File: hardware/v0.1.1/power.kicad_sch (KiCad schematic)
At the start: 5 parts

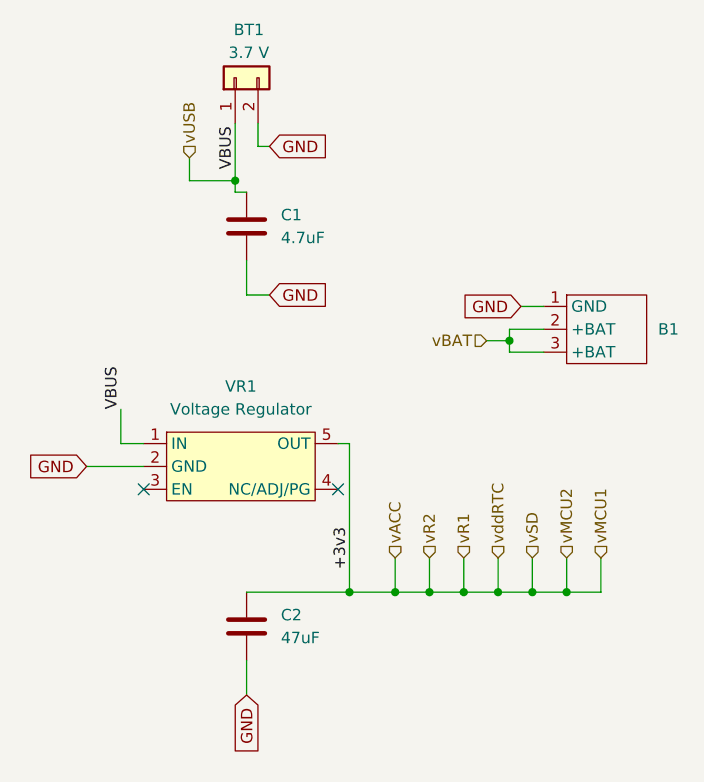
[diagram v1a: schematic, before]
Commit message: Pin updates and power fixes
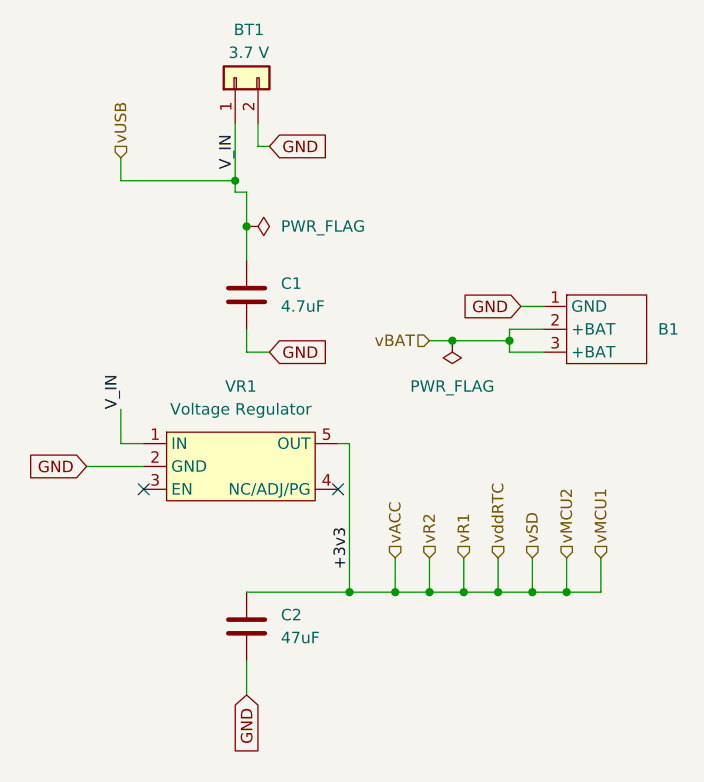
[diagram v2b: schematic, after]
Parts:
- VR1: symbol Device:Variable_Resistor -> PATCH_sym_2:Variable_Resistor
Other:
- moved on the sheet: C1
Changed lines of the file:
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@@
+	)
+	(junction
+		(at 165.1 93.98)
+		(diameter 0)
+		(color 0 0 0 0)
 	)
 	(junction
@@
 	)
 	(junction
+		(at 142.24 81.28)
+		(diameter 0)
+		(color 0 0 0 0)
+	)
+	(junction
 		(at 171.45 93.98)
 		(diameter 0)
@@
 	(wire
 		(pts
-			(xy 168.91 93.98) (xy 171.45 93.98)
-		)
-		(stroke
-			(width 0)
-			(type default)
-		)
-	)
-	(wire
-		(pts
-			(xy 142.24 88.9) (xy 144.78 88.9)
+			(xy 165.1 93.98) (xy 171.45 93.98)
 		)
 		(stroke
@@
 	(wire
 		(pts
+			(xy 142.24 81.28) (xy 142.24 85.09)
+		)
+		(stroke
+			(width 0)
+			(type default)
+		)
+	)
+	(wire
+		(pts
 			(xy 171.45 92.71) (xy 175.26 92.71)
 		)
@@
 	(wire
 		(pts
-			(xy 135.89 76.2) (xy 140.97 76.2)
-		)
-		(stroke
-			(width 0)
-			(type default)
-		)
-	)
-	(wire
-		(pts
 			(xy 170.18 118.11) (xy 170.18 121.92)
 		)
@@
 	(wire
 		(pts
+			(xy 142.24 95.25) (xy 144.78 95.25)
+		)
+		(stroke
+			(width 0)
+			(type default)
+		)
+	)
+	(wire
+		(pts
 			(xy 128.27 101.6) (xy 128.27 105.41)
 		)
@@
 	(wire
 		(pts
+			(xy 142.24 77.47) (xy 142.24 81.28)
+		)
+		(stroke
+			(width 0)
+			(type default)
+		)
+	)
+	(wire
+		(pts
 			(xy 177.8 121.92) (xy 181.61 121.92)
 		)
@@
 	(wire
 		(pts
+			(xy 128.27 76.2) (xy 140.97 76.2)
+		)
+		(stroke
+			(width 0)
+			(type default)
+		)
+	)
+	(wire
+		(pts
 			(xy 171.45 95.25) (xy 171.45 93.98)
 		)
@@
 	(wire
 		(pts
-			(xy 135.89 73.66) (xy 135.89 76.2)
-		)
-		(stroke
-			(width 0)
-			(type default)
-		)
-	)
-	(wire
-		(pts
 			(xy 171.45 93.98) (xy 171.45 92.71)
 		)
@@
 	(wire
 		(pts
-			(xy 142.24 85.09) (xy 142.24 88.9)
-		)
-		(stroke
-			(width 0)
-			(type default)
-		)
-	)
-	(wire
-		(pts
 			(xy 181.61 118.11) (xy 181.61 121.92)
 		)
@@
 	(wire
 		(pts
+			(xy 128.27 76.2) (xy 128.27 73.66)
+		)
+		(stroke
+			(width 0)
+			(type default)
+		)
+	)
+	(wire
+		(pts
 			(xy 143.51 69.85) (xy 143.51 72.39)
 		)
@@
 	(wire
 		(pts
+			(xy 162.56 93.98) (xy 165.1 93.98)
+		)
+		(stroke
+			(width 0)
+			(type default)
+		)
+	)
+	(wire
+		(pts
 			(xy 177.8 118.11) (xy 177.8 121.92)
 		)
@@
 	(wire
 		(pts
+			(xy 142.24 92.71) (xy 142.24 95.25)
+		)
+		(stroke
+			(width 0)
+			(type default)
+		)
+	)
+	(wire
+		(pts
 			(xy 140.97 77.47) (xy 142.24 77.47)
 		)
@@
 		)
 	)
-	(label "VBUS"
+	(label "V_IN"
 		(at 140.97 74.93 90)
 		(effects
@@
 		)
 	)
-	(label "VBUS"
+	(label "V_IN"
 		(at 128.27 101.6 90)
 		(effects
@@
 	(global_label "GND"
 		(shape input)
-		(at 144.78 88.9 0)
+		(at 144.78 95.25 0)
 		(fields_autoplaced yes)
 		(effects
@@
 		)
 		(property "Intersheetrefs" "${INTERSHEET_REFS}"
-			(at 151.6357 88.9 0)
+			(at 151.6357 95.25 0)
 			(hide yes)
 			(show_name no)
@@
 	(hierarchical_label "vUSB"
 		(shape input)
-		(at 135.89 73.66 90)
+		(at 128.27 73.66 90)
 		(effects
 			(font
@@
 	(hierarchical_label "vBAT"
 		(shape input)
-		(at 168.91 93.98 180)
+		(at 162.56 93.98 180)
 		(effects
 			(font
@@
 	)
 	(symbol
+		(lib_id "power:PWR_FLAG")
+		(at 142.24 81.28 270)
+		(unit 1)
+		(body_style 1)
+		(exclude_from_sim no)
+		(in_bom yes)
+		(on_board yes)
+		(in_pos_files yes)
+		(dnp no)
+		(fields_autoplaced yes)
+		(property "Reference" "#FLG02"
+			(at 144.145 81.28 0)
+			(hide yes)
+			(show_name no)
+			(do_not_autoplace no)
+			(effects
+				(font
+					(size 1.27 1.27)
+				)
+			)
+		)
+		(property "Value" "PWR_FLAG"
+			(at 146.05 81.2799 90)
+			(show_name no)
+			(do_not_autoplace no)
+			(effects
+				(font
+					(size 1.27 1.27)
+				)
+				(justify left)
+			)
+		)
+		(property "Footprint" ""
+			(at 142.24 81.28 0)
+			(hide yes)
+			(show_name no)
+			(do_not_autoplace no)
+			(effects
+				(font
+					(size 1.27 1.27)
+				)
+			)
+		)
+		(property "Datasheet" ""
+			(at 142.24 81.28 0)
+			(hide yes)
+			(show_name no)
+			(do_not_autoplace no)
+			(effects
+				(font
+					(size 1.27 1.27)
+				)
+			)
+		)
+		(property "Description" "Special symbol for telling ERC where power comes from"
+			(at 142.24 81.28 0)
+			(hide yes)
+			(show_name no)
+			(do_not_autoplace no)
+			(effects
+				(font
+					(size 1.27 1.27)
+				)
+			)
+		)
+		(pin "1"
+		)
+		(instances
+			(project "v0.1.1"
+				(path "/7a79fc3a-eeb6-4250-8945-98f32aee51db/1d65f6b7-6fff-4119-b784-9bbaa5726a6f"
+					(reference "#FLG02")
+					(unit 1)
+				)
+			)
+		)
+	)
+	(symbol
 		(lib_id "Device:C")
 		(at 142.24 125.73 0)
@@
 	(symbol
 		(lib_id "Device:C")
-		(at 142.24 81.28 0)
+		(at 142.24 88.9 0)
 		(unit 1)
 		(body_style 1)
@@
 		(dnp no)
 		(property "Reference" "C1"
-			(at 146.05 80.0099 0)
+			(at 146.05 87.6299 0)
 			(show_name no)
 			(do_not_autoplace no)
@@
 		)
 		(property "Value" "4.7uF"
-			(at 146.05 82.5499 0)
+			(at 146.05 90.1699 0)
 			(show_name no)
 			(do_not_autoplace no)
@@
 		)
 		(property "Footprint" "Capacitor_SMD:C_0603_1608Metric"
-			(at 143.2052 85.09 0)
+			(at 143.2052 92.71 0)
 			(hide yes)
 			(show_name no)
@@
 		)
 		(property "Datasheet" "https://mm.digikey.com/Volume0/opasdata/d220001/medias/docus/609/CL10A475KP8NNNC_Spec.pdf"
-			(at 142.24 81.28 0)
+			(at 142.24 88.9 0)
 			(hide yes)
 			(show_name no)
@@
 		)
 		(property "Description" "CL10A475KP8NNNC"
-			(at 142.24 81.28 0)
+			(at 142.24 88.9 0)
 			(hide yes)
 			(show_name no)
@@
 	)
 	(symbol
-		(lib_id "Device:Variable_Resistor")
+		(lib_id "power:PWR_FLAG")
+		(at 165.1 93.98 180)
+		(unit 1)
+		(body_style 1)
+		(exclude_from_sim no)
+		(in_bom yes)
+		(on_board yes)
+		(in_pos_files yes)
+		(dnp no)
+		(fields_autoplaced yes)
+		(property "Reference" "#FLG01"
+			(at 165.1 95.885 0)
+			(hide yes)
+			(show_name no)
+			(do_not_autoplace no)
+			(effects
+				(font
+					(size 1.27 1.27)
+				)
+			)
+		)
+		(property "Value" "PWR_FLAG"
+			(at 165.1 99.06 0)
+			(show_name no)
+			(do_not_autoplace no)
+			(effects
+				(font
+					(size 1.27 1.27)
+				)
+			)
+		)
+		(property "Footprint" ""
+			(at 165.1 93.98 0)
+			(hide yes)
+			(show_name no)
+			(do_not_autoplace no)
+			(effects
+				(font
+					(size 1.27 1.27)
+				)
+			)
+		)
+		(property "Datasheet" ""
+			(at 165.1 93.98 0)
+			(hide yes)
+			(show_name no)
+			(do_not_autoplace no)
+			(effects
+				(font
+					(size 1.27 1.27)
+				)
+			)
+		)
+		(property "Description" "Special symbol for telling ERC where power comes from"
+			(at 165.1 93.98 0)
+			(hide yes)
+			(show_name no)
+			(do_not_autoplace no)
+			(effects
+				(font
+					(size 1.27 1.27)
+				)
+			)
+		)
+		(pin "1"
+		)
+		(instances
+			(project "v0.1.1"
+				(path "/7a79fc3a-eeb6-4250-8945-98f32aee51db/1d65f6b7-6fff-4119-b784-9bbaa5726a6f"
+					(reference "#FLG01")
+					(unit 1)
+				)
+			)
+		)
+	)
+	(symbol
+		(lib_id "PATCH_sym_2:Variable_Resistor")
 		(at 138.43 104.14 0)
 		(unit 1)
